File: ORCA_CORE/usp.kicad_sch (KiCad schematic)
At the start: 15 parts, among them U11 AP64502

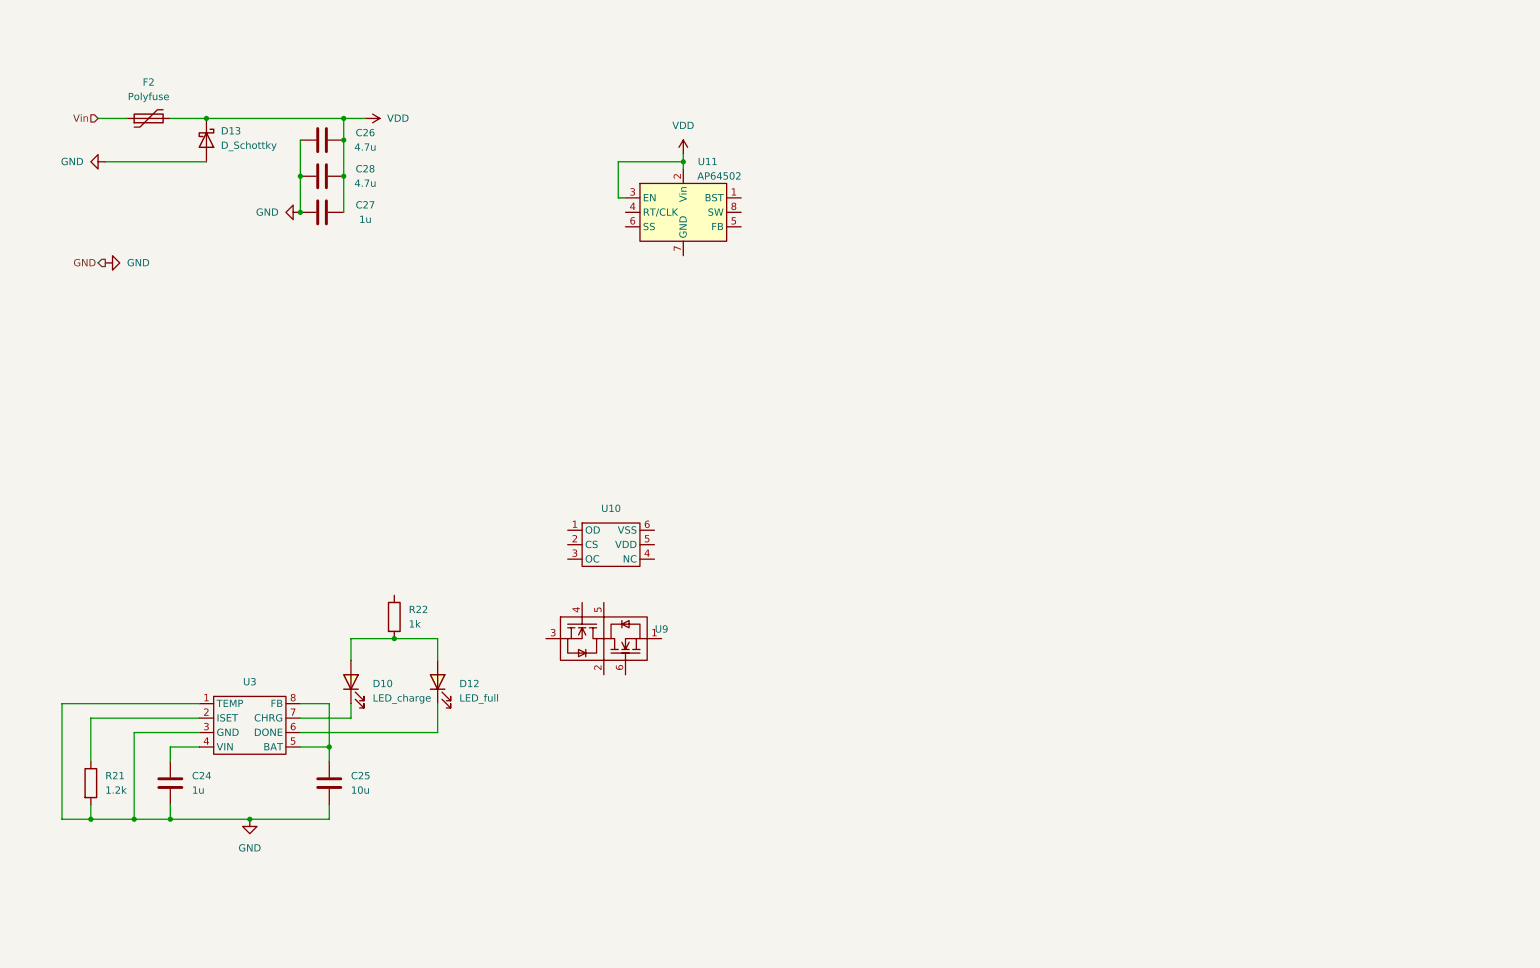
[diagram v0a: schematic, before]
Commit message: made usp (sketch only)
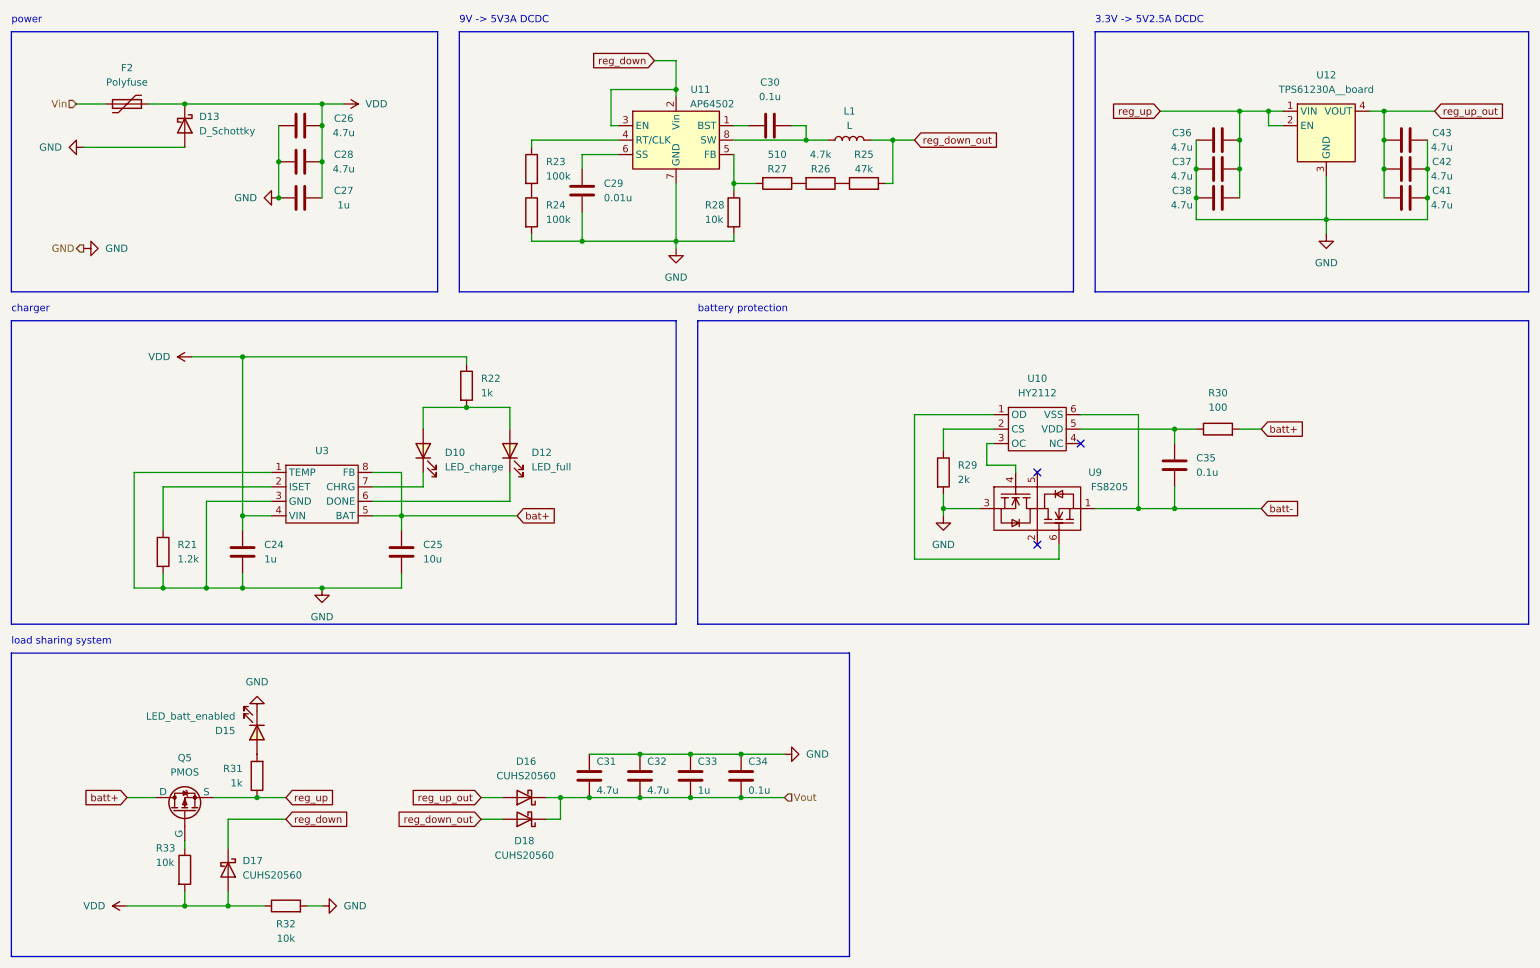
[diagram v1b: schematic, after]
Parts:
- added C29: 0.01u, symbol Device:C
- added C30, C34, C35: 0.1u, symbol Device:C
- added C31, C32, C36, C37, C38, C41, C42, C43: 4.7u, symbol Device:C
- added C33: 1u, symbol Device:C
- added D15: LED_batt_enabled, symbol Device:LED_Filled
- added D16, D17, D18: CUHS20560, symbol Device:D_Schottky
- added L1: L, symbol Device:L
- added Q5: PMOS, symbol Simulation_SPICE:PMOS
- added R23, R24: 100k, symbol Device:R
- added R25: 47k, symbol Device:R
- added R26: 4.7k, symbol Device:R
- added R27: 510, symbol Device:R
- added R28, R32, R33: 10k, symbol Device:R
- added R29: 2k, symbol Device:R
- added R30: 100, symbol Device:R
- added R31: 1k, symbol Device:R
- added U12: TPS61230A__board, symbol mylib:TPS61230A_board
- U10: value ~ -> HY2112
- U9: value ~ -> FS8205
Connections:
- net GND: now also U11.7 (GND), U11.9 (PAD), U9.3, C29.2, C31.1, C32.1, C33.1, C34.1, C36.1, C37.1, C38.1, C41.1, C42.1, C43.1, D15.1 (K), R24.2, R28.2, R29.2, R32.2, U12.3 (GND), U12.5 (GND)
- net VDD: now also C24.1, R22.1, U3.4 (VIN), D17.2 (A), R32.1, R33.2; no longer U11.2 (Vin), U11.3 (EN)
- net bat+: now reaches C25.1, U3.5 (BAT), U3.8 (FB)
- net at U10.1 (OD): now also U9.6
- net at U10.2 (CS): now also R29.1
- net at U10.3 (OC): now also U9.4
- net at U10.5 (VDD): now also C35.1, R30.1
- net batt-: now reaches U10.6 (VSS)
- net batt-: now also U9.1, C35.2
- net at U11.1 (BST): now also C30.2
- net at U11.4 (RT/CLK): now also R23.1
- net at U11.5 (FB): now also R27.2, R28.1
- net at U11.6 (SS): now also C29.1
- net at U11.8 (SW): now also C30.1, L1.1
- new net: Q5.2 (G), R33.1
- new net: R23.2, R24.1
- new net: D15.2 (A), R31.2
- new net: R25.1, R26.1
- new net: R26.2, R27.1
- new net Vout: C31.2, C32.2, C33.2, C34.2, D16.1 (K), D18.1 (K)
- new net batt+: Q5.1 (D), R30.2
- new net reg_down: D17.1 (K), U11.2 (Vin), U11.3 (EN)
- new net reg_down_out: D18.2 (A), L1.2, R25.2
- new net reg_up: C36.2, C37.2, C38.2, Q5.3 (S), R31.1, U12.1 (VIN), U12.2 (EN)
- new net reg_up_out: C41.2, C42.2, C43.2, D16.2 (A), U12.4 (VOUT)
- no-connect marks 0 -> 3
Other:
- note added: "3.3V -> 5V2.5A DCDC"
- note added: "9V -> 5V3A DCDC"
- note added: "battery protection"
- note added: "charger"
- note added: "load sharing system"
- note added: "power"
- moved on the sheet: C24, C25, C26, C27, C28, D10, D12, D13, F2, R21, R22, U10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
